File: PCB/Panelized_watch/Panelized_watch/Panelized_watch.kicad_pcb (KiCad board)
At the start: 4 copper layers, 90 x 51 mm, 276 parts, among them J1 Conn_01x06_Socket, J2 USB_C_Receptacle_PowerOnly_6P, Q1 BC817, Q2 AO3400A, SW1 SW_DPST_x2, SW2 SW_DPST_x2, SW3 SW_DPST_x2, U1 BH1750FVI-TR, U2 74AHCT1G125, U3 STM32L031G6Ux, U4 LP5912-3.3DRV, U5 MCP73831-3-OT, U6 MT3608, Y1 32.768kHz

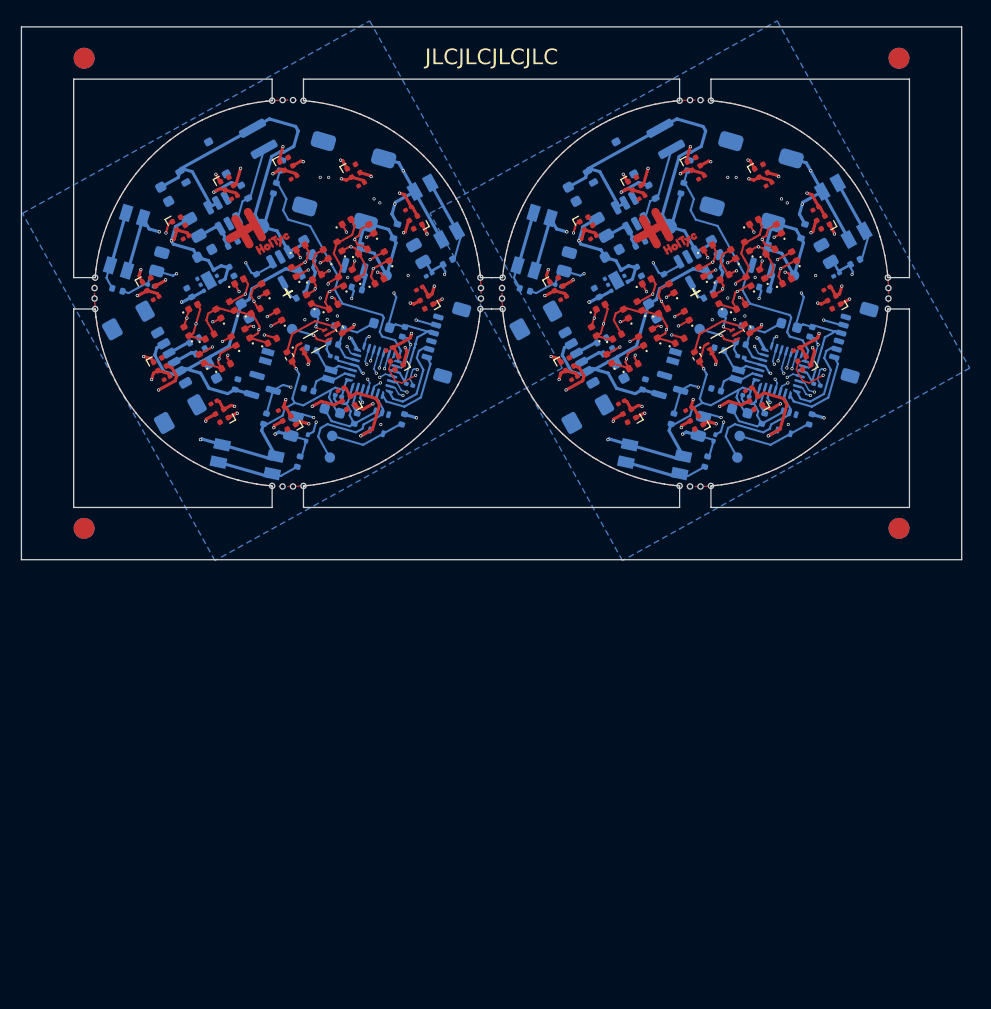
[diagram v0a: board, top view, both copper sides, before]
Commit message: Revision.B.0
Production folder in panelized_watch was send to production. YAAAH
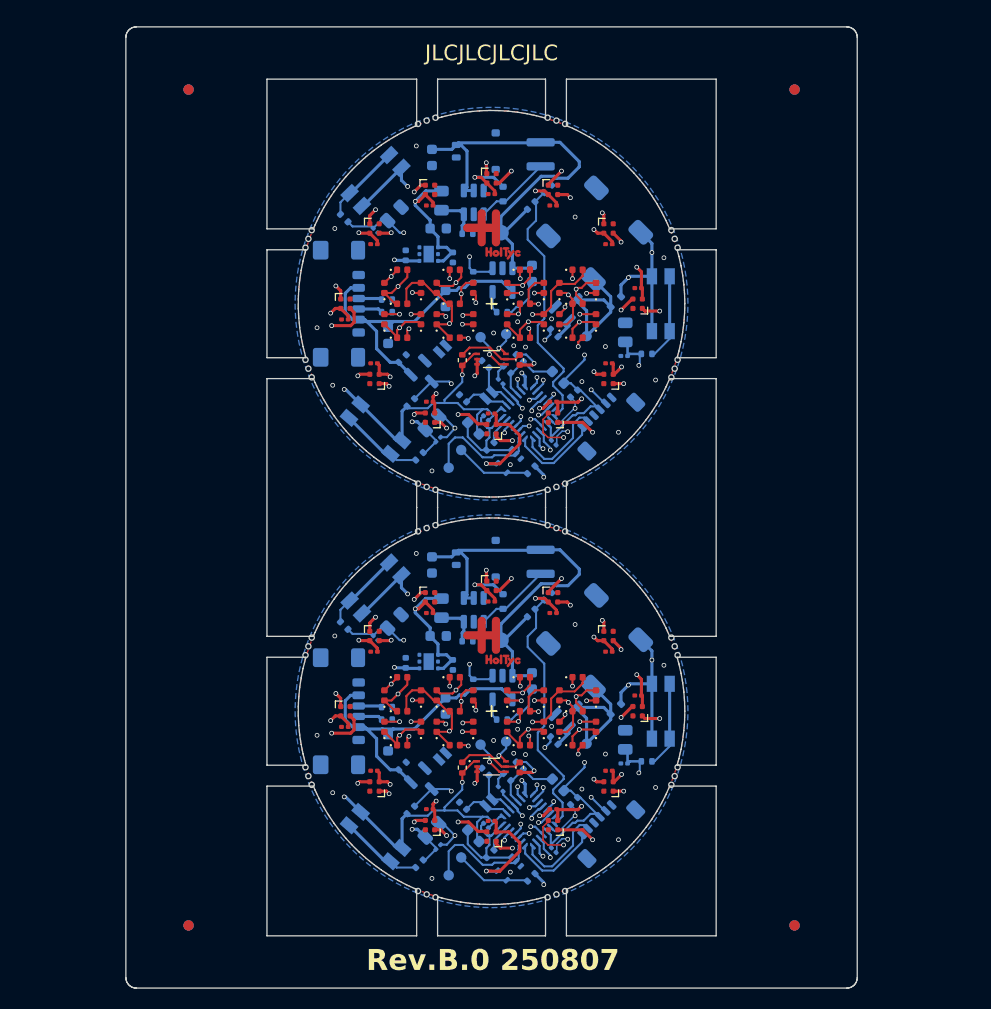
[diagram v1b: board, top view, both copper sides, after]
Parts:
- removed the BAT at (126.5, 39.1)
- removed the BAT at (165.5, 39.1)
- removed the BUZ at (138.5, 43.8)
- removed the BUZ at (177.5, 43.8)
- removed the BZ1 at (173.4, 34.8)
- removed the BZ1 at (134.4, 34.8)
- removed the C1 at (154.9, 44.8)
- removed the C1 at (115.9, 44.8)
- removed the C10 at (179.1, 49.2)
- removed the C10 at (140.1, 49.2)
- removed the C11 at (133.4, 51.6)
- removed the C11 at (172.4, 51.6)
- removed the C12 at (170.0, 54.7)
- removed the C12 at (131.0, 54.7)
- removed the C13 at (170.3, 50.8)
- removed the C13 at (131.3, 50.8)
- removed the C14 at (162.9, 36.3)
- removed the C14 at (123.9, 36.3)
- removed the C15 at (129.6, 34.4)
- removed the C15 at (168.6, 34.4)
- removed the C16 at (175.1, 35.1)
- removed the C16 at (136.1, 35.1)
- removed the C17 at (179.5, 37.4)
- removed the C17 at (140.5, 37.4)
- removed the C18 at (141.6, 45.0)
- removed the C18 at (180.6, 45.0)
- removed the C19 at (177.7, 50.8)
- removed the C19 at (138.7, 50.8)
- removed the C2 at (134.0, 48.9)
- removed the C2 at (173.0, 48.9)
- removed the C20 at (134.1, 54.7)
- removed the C20 at (173.1, 54.7)
- removed the C21 at (128.4, 56.6)
- removed the C21 at (167.4, 56.6)
- removed the C22 at (160.9, 55.9)
- removed the C22 at (121.9, 55.9)
- removed the C23 at (156.4, 53.6)
- removed the C23 at (117.4, 53.6)
- removed the C24 at (116.4, 46.0)
- removed the C24 at (155.4, 46.0)
- removed the C25 at (119.3, 40.1)
- removed the C25 at (158.3, 40.1)
- removed the C26 at (160.8, 52.9)
- removed the C26 at (121.8, 52.9)
- removed the C27 at (162.6, 43.4)
- removed the C27 at (123.6, 43.4)
- removed the C28 at (119.6, 45.4)
- removed the C28 at (158.6, 45.4)
- removed the C29 at (124.9, 47.2)
- removed the C29 at (163.9, 47.2)
- removed the C3 at (130.8, 59.3)
- removed the C3 at (169.8, 59.3)
- removed the C30 at (130.9, 41.1)
- removed the C30 at (169.9, 41.1)
- removed the C31 at (121.0, 41.7)
- removed the C31 at (160.0, 41.7)
- removed the C32 at (117.2, 36.0)
- removed the C32 at (156.2, 36.0)
- removed the C4 at (142.5, 43.7)
- removed the C4 at (181.5, 43.7)
- removed the C5 at (172.3, 56.8)
- removed the C5 at (133.3, 56.8)
- removed the C6 at (172.8, 55.3)
- removed the C6 at (133.8, 55.3)
- removed the C7 at (179.6, 54.2)
- removed the C7 at (140.6, 54.2)
- removed the C8 at (172.4, 50.3)
- removed the C8 at (133.4, 50.3)
- removed the C9 at (172.9, 48.7)
- removed the C9 at (133.9, 48.7)
- removed the D1 at (162.2, 35.0)
- removed the D1 at (123.2, 35.0)
- removed the D10 at (116.8, 52.3)
- removed the D10 at (155.8, 52.3)
- removed the D11 at (154.7, 44.6)
- removed the D11 at (115.7, 44.6)
- removed the D12 at (118.6, 38.8)
- removed the D12 at (157.6, 38.8)
- removed the D13 at (158.9, 46.8)
- removed the D13 at (119.9, 46.8)
- removed the D14 at (122.4, 47.4)
- removed the D14 at (161.4, 47.4)
- removed the D15 at (162.8, 50.1)
- removed the D15 at (123.8, 50.1)
- removed the D16 at (162.1, 52.5)
- removed the D16 at (123.1, 52.5)
- removed the D17 at (120.8, 51.8)
- removed the D17 at (159.8, 51.8)
- removed the D18 at (158.3, 49.1)
- removed the D18 at (119.3, 49.1)
- removed the D19 at (160.5, 49.6)
- removed the D19 at (121.5, 49.6)
- removed the D2 at (128.9, 33.1)
- removed the D2 at (167.9, 33.1)
- removed the D20 at (124.3, 44.4)
- removed the D20 at (163.3, 44.4)
- removed the D21 at (165.7, 45.0)
- removed the D21 at (126.7, 45.0)
- removed the D22 at (167.2, 47.6)
- removed the D22 at (128.2, 47.6)
- removed the D23 at (166.5, 50.0)
- removed the D23 at (127.5, 50.0)
- removed the D24 at (164.1, 49.3)
- removed the D24 at (125.1, 49.3)
- removed the D25 at (123.7, 46.7)
- removed the D25 at (162.7, 46.7)
- removed the D26 at (164.9, 47.2)
- removed the D26 at (125.9, 47.2)
- removed the D27 at (169.2, 41.1)
- removed the D27 at (130.2, 41.1)
- removed the D28 at (132.6, 41.7)
- removed the D28 at (171.6, 41.7)
- removed the D29 at (173.1, 44.4)
- removed the D29 at (134.1, 44.4)
- removed the D3 at (174.3, 33.8)
- removed the D3 at (135.3, 33.8)
- removed the D30 at (133.4, 46.8)
- removed the D30 at (172.4, 46.8)
- removed the D31 at (170.0, 46.1)
- removed the D31 at (131.0, 46.1)
- removed the D32 at (129.6, 43.5)
- removed the D32 at (168.6, 43.5)
- removed the D33 at (170.8, 43.9)
- removed the D33 at (131.8, 43.9)
- removed the D34 at (134.6, 38.7)
- removed the D34 at (173.6, 38.7)
- removed the D35 at (137.0, 39.3)
- removed the D35 at (176.0, 39.3)
- removed the D36 at (177.5, 41.9)
- removed the D36 at (138.5, 41.9)
- removed the D37 at (176.8, 44.3)
- removed the D37 at (137.8, 44.3)
- removed the D38 at (135.4, 43.6)
- removed the D38 at (174.4, 43.6)
- removed the D39 at (172.9, 41.0)
- removed the D39 at (133.9, 41.0)
- removed the D4 at (141.2, 38.7)
- removed the D4 at (180.2, 38.7)
- removed the D40 at (136.2, 41.5)
- removed the D40 at (175.2, 41.5)
- removed the D43 at (178.3, 39.6)
- removed the D43 at (139.3, 39.6)
- removed the D45 at (124.9, 35.8)
- removed the D45 at (163.9, 35.8)
- removed the D5 at (142.3, 46.4)
- removed the D5 at (181.3, 46.4)
- removed the D6 at (178.4, 52.2)
- removed the D6 at (139.4, 52.2)
- removed the D7 at (173.8, 56.0)
- removed the D7 at (134.8, 56.0)
- removed the D8 at (129.1, 57.9)
- removed the D8 at (168.1, 57.9)
- removed the D9 at (161.7, 57.2)
- removed the D9 at (122.7, 57.2)
- removed the DINL at (172.2, 59.1)
- removed the DINL at (133.2, 59.1)
- removed the DINS at (172.0, 61.2)
- removed the DINS at (133.0, 61.2)
- removed the FB1 at (177.0, 48.6)
- removed the FB1 at (138.0, 48.6)
- removed the J1 at (183.0, 50.0)
- removed the J1 at (144.0, 50.0)
- removed the J2 at (115.2, 53.1)
- removed the J2 at (154.2, 53.1)
- removed KiKit_MB_1_1, KiKit_MB_1_2, KiKit_MB_1_3, KiKit_MB_2_1, KiKit_MB_2_2, KiKit_MB_2_3, KiKit_MB_3_1, KiKit_MB_3_2, KiKit_MB_3_3, KiKit_MB_4_1, KiKit_MB_4_2, KiKit_MB_4_3, KiKit_MB_5_1, KiKit_MB_5_2, KiKit_MB_5_3, KiKit_MB_6_1, KiKit_MB_6_2, KiKit_MB_6_3, KiKit_MB_7_1, KiKit_MB_7_2, KiKit_MB_7_3, KiKit_MB_8_1, KiKit_MB_8_2, KiKit_MB_8_3: NPTH, NPTH
- removed the L1 at (165.2, 30.7)
- removed the L1 at (126.2, 30.7)
- removed the Li-po1 at (120.6, 33.5)
- removed the Li-po1 at (159.6, 33.5)
- removed the Q1 at (135.6, 42.2)
- removed the Q1 at (174.6, 42.2)
- removed the Q2 at (165.7, 54.5)
- removed the Q2 at (126.7, 54.5)
- removed the R10 at (174.5, 57.5)
- removed the R10 at (135.5, 57.5)
- removed the R11 at (179.0, 57.6)
- removed the R11 at (140.0, 57.6)
- removed the R13 at (166.8, 35.4)
- removed the R13 at (127.8, 35.4)
- removed the R14 at (167.4, 33.3)
- removed the R14 at (128.4, 33.3)
- removed the R15 at (120.6, 51.1)
- removed the R15 at (159.6, 51.1)
- removed the R16 at (120.0, 50.0)
- removed the R16 at (159.0, 50.0)
- removed the R17 at (126.8, 57.5)
- removed the R17 at (165.8, 57.5)
- removed the R18 at (159.0, 39.2)
- removed the R18 at (120.0, 39.2)
- removed the R19 at (169.3, 45.7)
- removed the R19 at (130.3, 45.7)
- removed the R20 at (163.1, 54.2)
- removed the R20 at (124.1, 54.2)
- removed the R21 at (165.2, 44.1)
- removed the R21 at (126.2, 44.1)
- removed the R22 at (123.7, 40.8)
- removed the R22 at (162.7, 40.8)
- removed the R23 at (129.2, 51.6)
- removed the R23 at (168.2, 51.6)
- removed the R3 at (116.7, 42.5)
- removed the R3 at (155.7, 42.5)
- removed the R4 at (112.7, 45.2)
- removed the R4 at (151.7, 45.2)
- removed the R5 at (168.5, 58.2)
- removed the R5 at (129.5, 58.2)
- removed the R6 at (169.0, 61.6)
- removed the R6 at (130.0, 61.6)
- removed the R7 at (141.5, 41.7)
- removed the R7 at (180.5, 41.7)
- removed the R8 at (174.6, 45.0)
- removed the R8 at (135.6, 45.0)
- removed the R9 at (183.3, 42.5)
- removed the R9 at (144.3, 42.5)
- removed the SCL at (131.6, 47.4)
- removed the SCL at (170.6, 47.4)
- removed the SDA at (168.4, 48.9)
- removed the SDA at (129.4, 48.9)
- removed the SW1 at (164.1, 61.4)
- removed the SW1 at (125.1, 61.4)
- removed the SW2 at (143.2, 37.6)
- removed the SW2 at (182.2, 37.6)
- removed the SW3 at (152.6, 40.6)
- removed the SW3 at (113.6, 40.6)
- removed the U1 at (131.6, 50.1)
- removed the U1 at (170.6, 50.1)
- removed the U2 at (176.8, 57.8)
- removed the U2 at (137.8, 57.8)
- removed the U3 at (137.2, 52.9)
- removed the U3 at (176.2, 52.9)
- removed the U4 at (121.4, 44.3)
- removed the U4 at (160.4, 44.3)
- removed the U5 at (128.8, 43.0)
- removed the U5 at (167.8, 43.0)
- removed the U6 at (161.8, 37.8)
- removed the U6 at (122.8, 37.8)
- removed the Y1 at (169.0, 52.4)
- removed the Y1 at (130.0, 52.4)
- added BAT: 2.7-4.2V, TestPoint:TestPoint_Pad_D1.5mm, B.Cu at (149.4, 39.7)
- added BAT: 2.7-4.2V, TestPoint:TestPoint_Pad_D1.5mm, B.Cu at (149.4, 78.7)
- added BUZ: ~, TestPoint:TestPoint_Pad_D1.0mm, B.Cu at (157.6, 49.6)
- added BUZ: ~, TestPoint:TestPoint_Pad_D1.0mm, B.Cu at (157.6, 88.6)
- added BZ1: Buzzer, Buzzer_SMD:Buzzer_SMD, B.Cu at (158.4, 39.8)
- added BZ1: Buzzer, Buzzer_SMD:Buzzer_SMD, B.Cu at (158.4, 78.8)
- added C1: 100n, Capacitor_SMD:C_0201_0603Metric, B.Cu at (137.4, 39.5)
- added C1: 100n, Capacitor_SMD:C_0201_0603Metric, B.Cu at (137.4, 78.5)
- added C10: 1u, Capacitor_SMD:C_0402_1005Metric, B.Cu at (156.4, 55.1)
- added C10: 1u, Capacitor_SMD:C_0402_1005Metric, B.Cu at (156.4, 94.1)
- added C11: 100n, Capacitor_SMD:C_0201_0603Metric, B.Cu at (149.4, 92.9)
- added C11: 100n, Capacitor_SMD:C_0201_0603Metric, B.Cu at (149.4, 53.9)
- added C12: 15pF, Capacitor_SMD:C_0402_1005Metric, B.Cu at (145.8, 94.5)
- added C12: 15pF, Capacitor_SMD:C_0402_1005Metric, B.Cu at (145.8, 55.5)
- added C13: 15pF, Capacitor_SMD:C_0402_1005Metric, B.Cu at (147.9, 52.3)
- added C13: 15pF, Capacitor_SMD:C_0402_1005Metric, B.Cu at (147.9, 91.3)
- added C14: 100n, Capacitor_SMD:C_0201_0603Metric, F.Cu at (148.5, 36.0)
- added C14: 100n, Capacitor_SMD:C_0201_0603Metric, F.Cu at (148.5, 75.0)
- added C15: 100n, Capacitor_SMD:C_0201_0603Metric, F.Cu at (154.4, 76.1)
- added C15: 100n, Capacitor_SMD:C_0201_0603Metric, F.Cu at (154.4, 37.1)
- added C16: 100n, Capacitor_SMD:C_0201_0603Metric, F.Cu at (159.7, 79.8)
- added C16: 100n, Capacitor_SMD:C_0201_0603Metric, F.Cu at (159.7, 40.8)
- added C17: 100n, Capacitor_SMD:C_0201_0603Metric, F.Cu at (162.5, 45.0)
- added C17: 100n, Capacitor_SMD:C_0201_0603Metric, F.Cu at (162.5, 84.0)
- added C18: 100n, Capacitor_SMD:C_0201_0603Metric, F.Cu at (159.7, 91.2)
- added C18: 100n, Capacitor_SMD:C_0201_0603Metric, F.Cu at (159.7, 52.2)
- added C19: 100n, Capacitor_SMD:C_0201_0603Metric, F.Cu at (154.4, 94.9)
- added C19: 100n, Capacitor_SMD:C_0201_0603Metric, F.Cu at (154.4, 55.9)
- added C2: 1u, Capacitor_SMD:C_0402_1005Metric, F.Cu at (151.2, 51.9)
- added C2: 1u, Capacitor_SMD:C_0402_1005Metric, F.Cu at (151.2, 90.9)
- added C20: 100n, Capacitor_SMD:C_0201_0603Metric, F.Cu at (148.5, 96.0)
- added C20: 100n, Capacitor_SMD:C_0201_0603Metric, F.Cu at (148.5, 57.0)
- added C21: 100n, Capacitor_SMD:C_0201_0603Metric, F.Cu at (142.6, 55.9)
- added C21: 100n, Capacitor_SMD:C_0201_0603Metric, F.Cu at (142.6, 94.9)
- added C22: 100n, Capacitor_SMD:C_0201_0603Metric, F.Cu at (137.3, 52.2)
- added C22: 100n, Capacitor_SMD:C_0201_0603Metric, F.Cu at (137.3, 91.2)
- added C23: 100n, Capacitor_SMD:C_0201_0603Metric, F.Cu at (134.5, 48.0)
- added C23: 100n, Capacitor_SMD:C_0201_0603Metric, F.Cu at (134.5, 87.0)
- added C24: 100n, Capacitor_SMD:C_0201_0603Metric, F.Cu at (137.3, 79.8)
- added C24: 100n, Capacitor_SMD:C_0201_0603Metric, F.Cu at (137.3, 40.8)
- added C25: 100n, Capacitor_SMD:C_0201_0603Metric, F.Cu at (142.6, 76.1)
- added C25: 100n, Capacitor_SMD:C_0201_0603Metric, F.Cu at (142.6, 37.1)
- added C26: 10u, Capacitor_SMD:C_0603_1608Metric, B.Cu at (138.6, 88.5)
- added C26: 10u, Capacitor_SMD:C_0603_1608Metric, B.Cu at (138.6, 49.5)
- added C27: 1u, Capacitor_SMD:C_0402_1005Metric, B.Cu at (144.8, 42.1)
- added C27: 1u, Capacitor_SMD:C_0402_1005Metric, B.Cu at (144.8, 81.1)
- added C28: 1u, Capacitor_SMD:C_0402_1005Metric, B.Cu at (140.3, 41.9)
- added C28: 1u, Capacitor_SMD:C_0402_1005Metric, B.Cu at (140.3, 80.9)
- added C29: 4.7uF, Capacitor_SMD:C_0603_1608Metric, B.Cu at (144.1, 85.0)
- added C29: 4.7uF, Capacitor_SMD:C_0603_1608Metric, B.Cu at (144.1, 46.0)
- added C3: 100n, Capacitor_SMD:C_0201_0603Metric, B.Cu at (143.4, 59.5)
- added C3: 100n, Capacitor_SMD:C_0201_0603Metric, B.Cu at (143.4, 98.5)
- added C30: 4.7uF, Capacitor_SMD:C_0603_1608Metric, B.Cu at (152.4, 82.6)
- added C30: 4.7uF, Capacitor_SMD:C_0603_1608Metric, B.Cu at (152.4, 43.6)
- added C31: 10u, Capacitor_SMD:C_0603_1608Metric, B.Cu at (143.4, 78.3)
- added C31: 10u, Capacitor_SMD:C_0603_1608Metric, B.Cu at (143.4, 39.3)
- added C32: 10u, Capacitor_SMD:C_0603_1608Metric, B.Cu at (142.8, 32.5)
- added C32: 10u, Capacitor_SMD:C_0603_1608Metric, B.Cu at (142.8, 71.5)
- added C4: 100n, Capacitor_SMD:C_0201_0603Metric, B.Cu at (161.2, 90.5)
- added C4: 100n, Capacitor_SMD:C_0201_0603Metric, B.Cu at (161.2, 51.5)
- added C5: 10u, Capacitor_SMD:C_0603_1608Metric, B.Cu at (146.8, 58.4)
- added C5: 10u, Capacitor_SMD:C_0603_1608Metric, B.Cu at (146.8, 97.4)
- added C6: 100n, Capacitor_SMD:C_0201_0603Metric, B.Cu at (148.0, 57.4)
- added C6: 100n, Capacitor_SMD:C_0201_0603Metric, B.Cu at (148.0, 96.4)
- added C7: 100n, Capacitor_SMD:C_0201_0603Metric, B.Cu at (154.4, 98.8)
- added C7: 100n, Capacitor_SMD:C_0201_0603Metric, B.Cu at (154.4, 59.8)
- added C8: 10n, Capacitor_SMD:C_0402_1005Metric, B.Cu at (150.0, 52.8)
- added C8: 10n, Capacitor_SMD:C_0402_1005Metric, B.Cu at (150.0, 91.8)
- added C9: 1u, Capacitor_SMD:C_0402_1005Metric, B.Cu at (151.2, 51.7)
- added C9: 1u, Capacitor_SMD:C_0402_1005Metric, B.Cu at (151.2, 90.7)
- added D1: SK6805, LED_SMD:LED_SK6812_EC15_1.5x1.5mm, F.Cu at (148.5, 34.5)
- added D1: SK6805, LED_SMD:LED_SK6812_EC15_1.5x1.5mm, F.Cu at (148.5, 73.5)
- added D10: SK6805, LED_SMD:LED_SK6812_EC15_1.5x1.5mm, F.Cu at (134.5, 46.5)
- added D10: SK6805, LED_SMD:LED_SK6812_EC15_1.5x1.5mm, F.Cu at (134.5, 85.5)
- added D11: SK6805, LED_SMD:LED_SK6812_EC15_1.5x1.5mm, F.Cu at (137.3, 39.3)
- added D11: SK6805, LED_SMD:LED_SK6812_EC15_1.5x1.5mm, F.Cu at (137.3, 78.3)
- added D12: SK6805, LED_SMD:LED_SK6812_EC15_1.5x1.5mm, F.Cu at (142.6, 35.6)
- added D12: SK6805, LED_SMD:LED_SK6812_EC15_1.5x1.5mm, F.Cu at (142.6, 74.6)
- added D13: LED, LED_SMD:LED_0402_1005Metric, F.Cu at (139.9, 82.2)
- added D13: LED, LED_SMD:LED_0402_1005Metric, F.Cu at (139.9, 43.2)
- added D14: LED, LED_SMD:LED_0402_1005Metric, F.Cu at (141.7, 84.0)
- added D14: LED, LED_SMD:LED_0402_1005Metric, F.Cu at (141.7, 45.0)
- added D15: LED, LED_SMD:LED_0402_1005Metric, F.Cu at (141.7, 87.0)
- added D15: LED, LED_SMD:LED_0402_1005Metric, F.Cu at (141.7, 48.0)
- added D16: LED, LED_SMD:LED_0402_1005Metric, F.Cu at (139.9, 49.7)
- added D16: LED, LED_SMD:LED_0402_1005Metric, F.Cu at (139.9, 88.7)
- added D17: LED, LED_SMD:LED_0402_1005Metric, F.Cu at (138.2, 48.0)
- added D17: LED, LED_SMD:LED_0402_1005Metric, F.Cu at (138.2, 87.0)
- added D18: LED, LED_SMD:LED_0402_1005Metric, F.Cu at (138.2, 84.0)
- added D18: LED, LED_SMD:LED_0402_1005Metric, F.Cu at (138.2, 45.0)
- added D19: LED, LED_SMD:LED_0402_1005Metric, F.Cu at (139.9, 46.5)
- added D19: LED, LED_SMD:LED_0402_1005Metric, F.Cu at (139.9, 85.5)
- added D2: SK6805, LED_SMD:LED_SK6812_EC15_1.5x1.5mm, F.Cu at (154.4, 74.6)
- added D2: SK6805, LED_SMD:LED_SK6812_EC15_1.5x1.5mm, F.Cu at (154.4, 35.6)
- added D20: LED, LED_SMD:LED_0402_1005Metric, F.Cu at (145.0, 43.2)
- added D20: LED, LED_SMD:LED_0402_1005Metric, F.Cu at (145.0, 82.2)
- added D21: LED, LED_SMD:LED_0402_1005Metric, F.Cu at (146.7, 45.0)
- added D21: LED, LED_SMD:LED_0402_1005Metric, F.Cu at (146.7, 84.0)
- added D22: LED, LED_SMD:LED_0402_1005Metric, F.Cu at (146.7, 87.0)
- added D22: LED, LED_SMD:LED_0402_1005Metric, F.Cu at (146.7, 48.0)
- added D23: LED, LED_SMD:LED_0402_1005Metric, F.Cu at (145.0, 49.7)
- added D23: LED, LED_SMD:LED_0402_1005Metric, F.Cu at (145.0, 88.7)
- added D24: LED, LED_SMD:LED_0402_1005Metric, F.Cu at (143.2, 48.0)
- added D24: LED, LED_SMD:LED_0402_1005Metric, F.Cu at (143.2, 87.0)
- added D25: LED, LED_SMD:LED_0402_1005Metric, F.Cu at (143.2, 84.0)
- added D25: LED, LED_SMD:LED_0402_1005Metric, F.Cu at (143.2, 45.0)
- added D26: LED, LED_SMD:LED_0402_1005Metric, F.Cu at (145.0, 46.5)
- added D26: LED, LED_SMD:LED_0402_1005Metric, F.Cu at (145.0, 85.5)
- added D27: LED, LED_SMD:LED_0402_1005Metric, F.Cu at (151.7, 82.2)
- added D27: LED, LED_SMD:LED_0402_1005Metric, F.Cu at (151.7, 43.2)
- added D28: LED, LED_SMD:LED_0402_1005Metric, F.Cu at (153.5, 45.0)
- added D28: LED, LED_SMD:LED_0402_1005Metric, F.Cu at (153.5, 84.0)
- added D29: LED, LED_SMD:LED_0402_1005Metric, F.Cu at (153.5, 48.0)
- added D29: LED, LED_SMD:LED_0402_1005Metric, F.Cu at (153.5, 87.0)
- added D3: SK6805, LED_SMD:LED_SK6812_EC15_1.5x1.5mm, F.Cu at (159.7, 78.3)
- added D3: SK6805, LED_SMD:LED_SK6812_EC15_1.5x1.5mm, F.Cu at (159.7, 39.3)
- added D30: LED, LED_SMD:LED_0402_1005Metric, F.Cu at (151.7, 88.7)
- added D30: LED, LED_SMD:LED_0402_1005Metric, F.Cu at (151.7, 49.7)
- added D31: LED, LED_SMD:LED_0402_1005Metric, F.Cu at (150.0, 48.0)
- added D31: LED, LED_SMD:LED_0402_1005Metric, F.Cu at (150.0, 87.0)
- added D32: LED, LED_SMD:LED_0402_1005Metric, F.Cu at (150.0, 84.0)
- added D32: LED, LED_SMD:LED_0402_1005Metric, F.Cu at (150.0, 45.0)
- added D33: LED, LED_SMD:LED_0402_1005Metric, F.Cu at (151.7, 85.5)
- added D33: LED, LED_SMD:LED_0402_1005Metric, F.Cu at (151.7, 46.5)
- added D34: LED, LED_SMD:LED_0402_1005Metric, F.Cu at (156.7, 43.2)
- added D34: LED, LED_SMD:LED_0402_1005Metric, F.Cu at (156.7, 82.2)
- added D35: LED, LED_SMD:LED_0402_1005Metric, F.Cu at (158.5, 84.0)
- added D35: LED, LED_SMD:LED_0402_1005Metric, F.Cu at (158.5, 45.0)
- added D36: LED, LED_SMD:LED_0402_1005Metric, F.Cu at (158.5, 87.0)
- added D36: LED, LED_SMD:LED_0402_1005Metric, F.Cu at (158.5, 48.0)
- added D37: LED, LED_SMD:LED_0402_1005Metric, F.Cu at (156.7, 88.7)
- added D37: LED, LED_SMD:LED_0402_1005Metric, F.Cu at (156.7, 49.7)
- added D38: LED, LED_SMD:LED_0402_1005Metric, F.Cu at (155.0, 48.0)
- added D38: LED, LED_SMD:LED_0402_1005Metric, F.Cu at (155.0, 87.0)
- added D39: LED, LED_SMD:LED_0402_1005Metric, F.Cu at (155.0, 84.0)
- added D39: LED, LED_SMD:LED_0402_1005Metric, F.Cu at (155.0, 45.0)
- added D4: SK6805, LED_SMD:LED_SK6812_EC15_1.5x1.5mm, F.Cu at (162.5, 85.5)
- added D4: SK6805, LED_SMD:LED_SK6812_EC15_1.5x1.5mm, F.Cu at (162.5, 46.5)
- added D40: LED, LED_SMD:LED_0402_1005Metric, F.Cu at (156.7, 46.5)
- added D40: LED, LED_SMD:LED_0402_1005Metric, F.Cu at (156.7, 85.5)
- added D43: D_Schottky, Diode_SMD:D_SOD-523, B.Cu at (160.4, 46.3)
- added D43: D_Schottky, Diode_SMD:D_SOD-523, B.Cu at (160.4, 85.3)
- added D45: D_Schottky, Diode_SMD:D_SOD-523, B.Cu at (149.6, 36.0)
- added D45: D_Schottky, Diode_SMD:D_SOD-523, B.Cu at (149.6, 75.0)
- added D5: SK6805, LED_SMD:LED_SK6812_EC15_1.5x1.5mm, F.Cu at (159.7, 92.7)
- added D5: SK6805, LED_SMD:LED_SK6812_EC15_1.5x1.5mm, F.Cu at (159.7, 53.7)
- added D6: SK6805, LED_SMD:LED_SK6812_EC15_1.5x1.5mm, F.Cu at (154.4, 57.4)
- added D6: SK6805, LED_SMD:LED_SK6812_EC15_1.5x1.5mm, F.Cu at (154.4, 96.4)
- added D7: SK6805, LED_SMD:LED_SK6812_EC15_1.5x1.5mm, F.Cu at (148.5, 97.5)
- added D7: SK6805, LED_SMD:LED_SK6812_EC15_1.5x1.5mm, F.Cu at (148.5, 58.5)
- added D8: SK6805, LED_SMD:LED_SK6812_EC15_1.5x1.5mm, F.Cu at (142.6, 57.4)
- added D8: SK6805, LED_SMD:LED_SK6812_EC15_1.5x1.5mm, F.Cu at (142.6, 96.4)
- added D9: SK6805, LED_SMD:LED_SK6812_EC15_1.5x1.5mm, F.Cu at (137.3, 92.7)
- added D9: SK6805, LED_SMD:LED_SK6812_EC15_1.5x1.5mm, F.Cu at (137.3, 53.7)
- added DINL: ~, TestPoint:TestPoint_Pad_D1.0mm, B.Cu at (145.6, 60.5)
- added DINL: ~, TestPoint:TestPoint_Pad_D1.0mm, B.Cu at (145.6, 99.5)
- added DINS: ~, TestPoint:TestPoint_Pad_D1.0mm, B.Cu at (144.4, 62.2)
- added DINS: ~, TestPoint:TestPoint_Pad_D1.0mm, B.Cu at (144.4, 101.2)
- added FB1: FerriteBead, Inductor_SMD:L_0603_1608Metric, B.Cu at (154.9, 53.5)
- added FB1: FerriteBead, Inductor_SMD:L_0603_1608Metric, B.Cu at (154.9, 92.5)
- added J1: Conn_01x06_Socket, Connector_JST:JST_SUR_SM06B-SURS-TF_1x06-1MP_P0.80mm_Horizontal, B.Cu at (159.4, 57.7)
- added J1: Conn_01x06_Socket, Connector_JST:JST_SUR_SM06B-SURS-TF_1x06-1MP_P0.80mm_Horizontal, B.Cu at (159.4, 96.7)
- added J2: USB_C_Receptacle_PowerOnly_6P, Connector_USB:USB_C_Receptacle_GCT_USB4135-GF-A_6P_TopMnt_Horizontal, B.Cu at (132.7, 46.5)
- added J2: USB_C_Receptacle_PowerOnly_6P, Connector_USB:USB_C_Receptacle_GCT_USB4135-GF-A_6P_TopMnt_Horizontal, B.Cu at (132.7, 85.5)
- added KiKit_MB_10_4: NPTH, NPTH, F.Cu at (131.3, 92.5)
- added KiKit_MB_10_5: NPTH, NPTH, F.Cu at (131.0, 91.7)
- added KiKit_MB_10_6: NPTH, NPTH, F.Cu at (130.7, 90.9)
- added KiKit_MB_11_4: NPTH, NPTH, F.Cu at (165.7, 78.5)
- added KiKit_MB_11_5: NPTH, NPTH, F.Cu at (166.0, 79.3)
- added KiKit_MB_11_6: NPTH, NPTH, F.Cu at (166.3, 80.1)
- added KiKit_MB_12_4: NPTH, NPTH, F.Cu at (166.3, 90.9)
- added KiKit_MB_12_5: NPTH, NPTH, F.Cu at (166.0, 91.7)
- added KiKit_MB_12_6: NPTH, NPTH, F.Cu at (165.7, 92.5)
- added KiKit_MB_13_4: NPTH, NPTH, F.Cu at (141.5, 68.3)
- added KiKit_MB_13_5: NPTH, NPTH, F.Cu at (142.3, 68.0)
- added KiKit_MB_13_6: NPTH, NPTH, F.Cu at (143.1, 67.7)
- added KiKit_MB_14_4: NPTH, NPTH, F.Cu at (153.9, 67.7)
- added KiKit_MB_14_5: NPTH, NPTH, F.Cu at (154.7, 68.0)
- added KiKit_MB_14_6: NPTH, NPTH, F.Cu at (155.5, 68.3)
- added KiKit_MB_15_4: NPTH, NPTH, F.Cu at (143.1, 103.3)
- added KiKit_MB_15_5: NPTH, NPTH, F.Cu at (142.3, 103.0)
- added KiKit_MB_15_6: NPTH, NPTH, F.Cu at (141.5, 102.7)
- added KiKit_MB_16_4: NPTH, NPTH, F.Cu at (155.5, 102.7)
- added KiKit_MB_16_5: NPTH, NPTH, F.Cu at (154.7, 103.0)
- added KiKit_MB_16_6: NPTH, NPTH, F.Cu at (153.9, 103.3)
- added KiKit_MB_1_5: NPTH, NPTH, F.Cu at (131.0, 40.3)
- added KiKit_MB_1_6: NPTH, NPTH, F.Cu at (131.3, 39.5)
- added KiKit_MB_2_5: NPTH, NPTH, F.Cu at (131.0, 52.7)
- added KiKit_MB_2_6: NPTH, NPTH, F.Cu at (130.7, 51.9)
- added KiKit_MB_3_5: NPTH, NPTH, F.Cu at (166.0, 40.3)
- added KiKit_MB_3_6: NPTH, NPTH, F.Cu at (166.3, 41.1)
- added KiKit_MB_4_5: NPTH, NPTH, F.Cu at (166.0, 52.7)
- added KiKit_MB_4_6: NPTH, NPTH, F.Cu at (165.7, 53.5)
- added KiKit_MB_5_5: NPTH, NPTH, F.Cu at (142.3, 29.0)
- added KiKit_MB_5_6: NPTH, NPTH, F.Cu at (143.1, 28.7)
- added KiKit_MB_6_5: NPTH, NPTH, F.Cu at (154.7, 29.0)
- added KiKit_MB_6_6: NPTH, NPTH, F.Cu at (155.5, 29.3)
- added KiKit_MB_7_5: NPTH, NPTH, F.Cu at (142.3, 64.0)
- added KiKit_MB_7_6: NPTH, NPTH, F.Cu at (141.5, 63.7)
- added KiKit_MB_8_5: NPTH, NPTH, F.Cu at (154.7, 64.0)
- added KiKit_MB_8_6: NPTH, NPTH, F.Cu at (153.9, 64.3)
- added KiKit_MB_9_4: NPTH, NPTH, F.Cu at (130.7, 80.1)
- added KiKit_MB_9_5: NPTH, NPTH, F.Cu at (131.0, 79.3)
- added KiKit_MB_9_6: NPTH, NPTH, F.Cu at (131.3, 78.5)
- added L1: 22uH, Inductor_SMD:L_Sunlord_SWPA3015S, B.Cu at (153.2, 71.2)
- added L1: 22uH, Inductor_SMD:L_Sunlord_SWPA3015S, B.Cu at (153.2, 32.2)
- added Li-po1: Conn_01x02_Socket, Connector_Molex:Molex_Pico-EZmate_78171-0002_1x02-1MP_P1.20mm_Vertical, B.Cu at (147.0, 31.9)
- added Li-po1: Conn_01x02_Socket, Connector_Molex:Molex_Pico-EZmate_78171-0002_1x02-1MP_P1.20mm_Vertical, B.Cu at (147.0, 70.9)
- added Q1: BC817, Package_TO_SOT_SMD:SOT-23, B.Cu at (155.9, 46.8)
- added Q1: BC817, Package_TO_SOT_SMD:SOT-23, B.Cu at (155.9, 85.8)
- added Q2: AO3400A, Package_TO_SOT_SMD:SOT-23, B.Cu at (142.1, 92.3)
- added Q2: AO3400A, Package_TO_SOT_SMD:SOT-23, B.Cu at (142.1, 53.3)
- added R10: 10K, Resistor_SMD:R_0402_1005Metric, B.Cu at (148.4, 99.1)
- added R10: 10K, Resistor_SMD:R_0402_1005Metric, B.Cu at (148.4, 60.1)
- added R11: 510, Resistor_SMD:R_0402_1005Metric, B.Cu at (152.3, 101.4)
- added R11: 510, Resistor_SMD:R_0402_1005Metric, B.Cu at (152.3, 62.4)
- added R13: 10K, Resistor_SMD:R_0402_1005Metric, B.Cu at (152.3, 76.1)
- added R13: 10K, Resistor_SMD:R_0402_1005Metric, B.Cu at (152.3, 37.1)
- added R14: 10K, Resistor_SMD:R_0402_1005Metric, B.Cu at (153.9, 35.5)
- added R14: 10K, Resistor_SMD:R_0402_1005Metric, B.Cu at (153.9, 74.5)
- added R15: 5K1, Resistor_SMD:R_0402_1005Metric, B.Cu at (138.5, 86.3)
- added R15: 5K1, Resistor_SMD:R_0402_1005Metric, B.Cu at (138.5, 47.3)
- added R16: 5K1, Resistor_SMD:R_0402_1005Metric, B.Cu at (138.5, 46.1)
- added R16: 5K1, Resistor_SMD:R_0402_1005Metric, B.Cu at (138.5, 85.1)
- added R17: 10K, Resistor_SMD:R_0402_1005Metric, B.Cu at (140.8, 94.9)
- added R17: 10K, Resistor_SMD:R_0402_1005Metric, B.Cu at (140.8, 55.9)
- added R18: 16.5K, Resistor_SMD:R_0805_2012Metric, B.Cu at (143.7, 75.6)
- added R18: 16.5K, Resistor_SMD:R_0805_2012Metric, B.Cu at (143.7, 36.6)
- added R19: 5K1, Resistor_SMD:R_0402_1005Metric, B.Cu at (149.5, 47.3)
- added R19: 5K1, Resistor_SMD:R_0402_1005Metric, B.Cu at (149.5, 86.3)
- added R20: 10K, Resistor_SMD:R_0402_1005Metric, B.Cu at (140.0, 51.7)
- added R20: 10K, Resistor_SMD:R_0402_1005Metric, B.Cu at (140.0, 90.7)
- added R21: 10k, Resistor_SMD:R_0402_1005Metric, B.Cu at (146.7, 43.9)
- added R21: 10k, Resistor_SMD:R_0402_1005Metric, B.Cu at (146.7, 82.9)
- added R22: 2.2K, Resistor_SMD:R_0402_1005Metric, B.Cu at (146.2, 39.8)
- added R22: 2.2K, Resistor_SMD:R_0402_1005Metric, B.Cu at (146.2, 78.8)
- added R23: 2.2K, Resistor_SMD:R_0402_1005Metric, F.Cu at (145.7, 90.9)
- added R23: 2.2K, Resistor_SMD:R_0402_1005Metric, F.Cu at (145.7, 51.9)
- added R3: 16.5K, Resistor_SMD:R_0805_2012Metric, B.Cu at (139.2, 76.9)
- added R3: 16.5K, Resistor_SMD:R_0805_2012Metric, B.Cu at (139.2, 37.9)
- added R4: 510, Resistor_SMD:R_0402_1005Metric, B.Cu at (134.4, 38.3)
- added R4: 510, Resistor_SMD:R_0402_1005Metric, B.Cu at (134.4, 77.3)
- added R5: 16.5K, Resistor_SMD:R_0805_2012Metric, B.Cu at (142.8, 57.9)
- added R5: 16.5K, Resistor_SMD:R_0805_2012Metric, B.Cu at (142.8, 96.9)
- added R6: 510, Resistor_SMD:R_0402_1005Metric, B.Cu at (141.6, 61.1)
- added R6: 510, Resistor_SMD:R_0402_1005Metric, B.Cu at (141.6, 100.1)
- added R7: 16.5K, Resistor_SMD:R_0805_2012Metric, B.Cu at (161.3, 88.2)
- added R7: 16.5K, Resistor_SMD:R_0805_2012Metric, B.Cu at (161.3, 49.2)
- added R8: 5K1, Resistor_SMD:R_0402_1005Metric, B.Cu at (154.5, 49.3)
- added R8: 5K1, Resistor_SMD:R_0402_1005Metric, B.Cu at (154.5, 88.3)
- added R9: 510, Resistor_SMD:R_0402_1005Metric, B.Cu at (163.3, 51.3)
- added R9: 510, Resistor_SMD:R_0402_1005Metric, B.Cu at (163.3, 90.3)
- added SCL: ~, TestPoint:TestPoint_Pad_D1.0mm, B.Cu at (149.9, 88.4)
- added SCL: ~, TestPoint:TestPoint_Pad_D1.0mm, B.Cu at (149.9, 49.4)
- added SDA: ~, TestPoint:TestPoint_Pad_D1.0mm, B.Cu at (147.4, 49.7)
- added SDA: ~, TestPoint:TestPoint_Pad_D1.0mm, B.Cu at (147.4, 88.7)
- added SW1: SW_DPST_x2, Button_Switch_SMD:Panasonic_EVQPUJ_EVQPUA, B.Cu at (137.4, 58.5)
- added SW1: SW_DPST_x2, Button_Switch_SMD:Panasonic_EVQPUJ_EVQPUA, B.Cu at (137.4, 97.5)
- added SW2: SW_DPST_x2, Button_Switch_SMD:Panasonic_EVQPUJ_EVQPUA, B.Cu at (164.7, 46.5)
- added SW2: SW_DPST_x2, Button_Switch_SMD:Panasonic_EVQPUJ_EVQPUA, B.Cu at (164.7, 85.5)
- added SW3: SW_DPST_x2, Button_Switch_SMD:Panasonic_EVQPUJ_EVQPUA, B.Cu at (137.4, 73.7)
- added SW3: SW_DPST_x2, Button_Switch_SMD:Panasonic_EVQPUJ_EVQPUA, B.Cu at (137.4, 34.7)
- added U1: BH1750FVI-TR, BH1750FVI-TR:XDCR_BH1750FVI-TR, F.Cu at (148.5, 51.8)
- added U1: BH1750FVI-TR, BH1750FVI-TR:XDCR_BH1750FVI-TR, F.Cu at (148.5, 90.8)
- added U2: 74AHCT1G125, Package_TO_SOT_SMD:SOT-353_SC-70-5, B.Cu at (150.2, 100.5)
- added U2: 74AHCT1G125, Package_TO_SOT_SMD:SOT-353_SC-70-5, B.Cu at (150.2, 61.5)
- added U3: STM32L031G6Ux, Package_DFN_QFN:QFN-28_4x4mm_P0.5mm, B.Cu at (152.1, 95.9)
- added U3: STM32L031G6Ux, Package_DFN_QFN:QFN-28_4x4mm_P0.5mm, B.Cu at (152.1, 56.9)
- added U4: LP5912-3.3DRV, Package_SON:WSON-6-1EP_2x2mm_P0.65mm_EP1x1.6mm, B.Cu at (142.5, 41.7)
- added U4: LP5912-3.3DRV, Package_SON:WSON-6-1EP_2x2mm_P0.65mm_EP1x1.6mm, B.Cu at (142.5, 80.7)
- added U5: MCP73831-3-OT, Package_TO_SOT_SMD:SOT-23-5, B.Cu at (149.5, 83.2)
- added U5: MCP73831-3-OT, Package_TO_SOT_SMD:SOT-23-5, B.Cu at (149.5, 44.2)
- added U6: MT3608, Package_TO_SOT_SMD:SOT-23-6, B.Cu at (146.8, 75.8)
- added U6: MT3608, Package_TO_SOT_SMD:SOT-23-6, B.Cu at (146.8, 36.8)
- added Y1: 32.768kHz, Crystal:Crystal_SMD_SeikoEpson_MC146-4Pin_6.7x1.5mm, B.Cu at (146.0, 92.0)
- added Y1: 32.768kHz, Crystal:Crystal_SMD_SeikoEpson_MC146-4Pin_6.7x1.5mm, B.Cu at (146.0, 53.0)
- moved KiKit_MB_7_4 45.6 mm to (143.1, 64.3)
- moved KiKit_MB_4_4 40.6 mm to (166.3, 51.9)
- moved KiKit_FID_B_4 39.3 mm to (177.5, 106.0)
- moved KiKit_FID_T_4 39.3 mm to (177.5, 106.0)
- moved KiKit_FID_B_3 39.3 mm to (119.5, 106.0)
- moved KiKit_FID_T_3 39.3 mm to (119.5, 106.0)
- moved KiKit_MB_6_4 37.4 mm to (153.9, 28.7)
- moved KiKit_MB_3_4 37.3 mm to (165.7, 39.5)
- moved KiKit_MB_1_4 20.3 mm to (130.7, 41.1)
- moved KiKit_MB_2_4 17.4 mm to (131.3, 53.5)
- moved KiKit_MB_5_4 16.8 mm to (141.5, 29.3)
- moved KiKit_MB_8_4 11.0 mm to (155.5, 63.7)
- moved KiKit_FID_B_2 10.4 mm to (177.5, 26.0)
- moved KiKit_FID_T_2 10.4 mm to (177.5, 26.0)
- moved KiKit_FID_B_1 10.4 mm to (119.5, 26.0)
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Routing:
- net Board_1-GND: track 30.3 -> 38.1 mm, vias 11 -> 16
- net Board_0-GND: track 30.3 -> 38.1 mm, vias 11 -> 16
- net Board_1-Row5: track 56.4 -> 50.5 mm, vias 7 -> 8
- net Board_0-Row5: track 56.4 -> 50.5 mm, vias 7 -> 8
- net Board_1-Net-(D5-DOUT): track 7.34 -> 12.9 mm
- net Board_0-Net-(D5-DOUT): track 7.34 -> 12.9 mm
- net Board_0-/NRST: track 13.5 -> 15.2 mm
- net Board_1-/NRST: track 13.5 -> 15.2 mm
- net Board_0-+5V: track 136.0 -> 137.6 mm
- net Board_1-+5V: track 136.0 -> 137.6 mm
- net Board_0-Net-(U1-DVI): track 8.06 -> 6.41 mm
- net Board_1-Net-(U1-DVI): track 8.06 -> 6.41 mm
- net Board_1-Net-(D1-DIN): track 41.3 -> 42.8 mm
- net Board_0-Net-(D1-DIN): track 41.3 -> 42.8 mm
- net Board_0-Button_R: track 18.1 -> 19.6 mm
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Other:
- board size 90 x 51 mm -> 70 x 92 mm
- board text added: "Rev.B.0 250807"
